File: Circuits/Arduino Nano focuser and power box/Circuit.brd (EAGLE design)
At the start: 67.4 x 71.6 mm, 30 parts, among them IC1 7805L, J2 RJ11, Q2 IRF540, Q3 IRF540, Q5 BC547

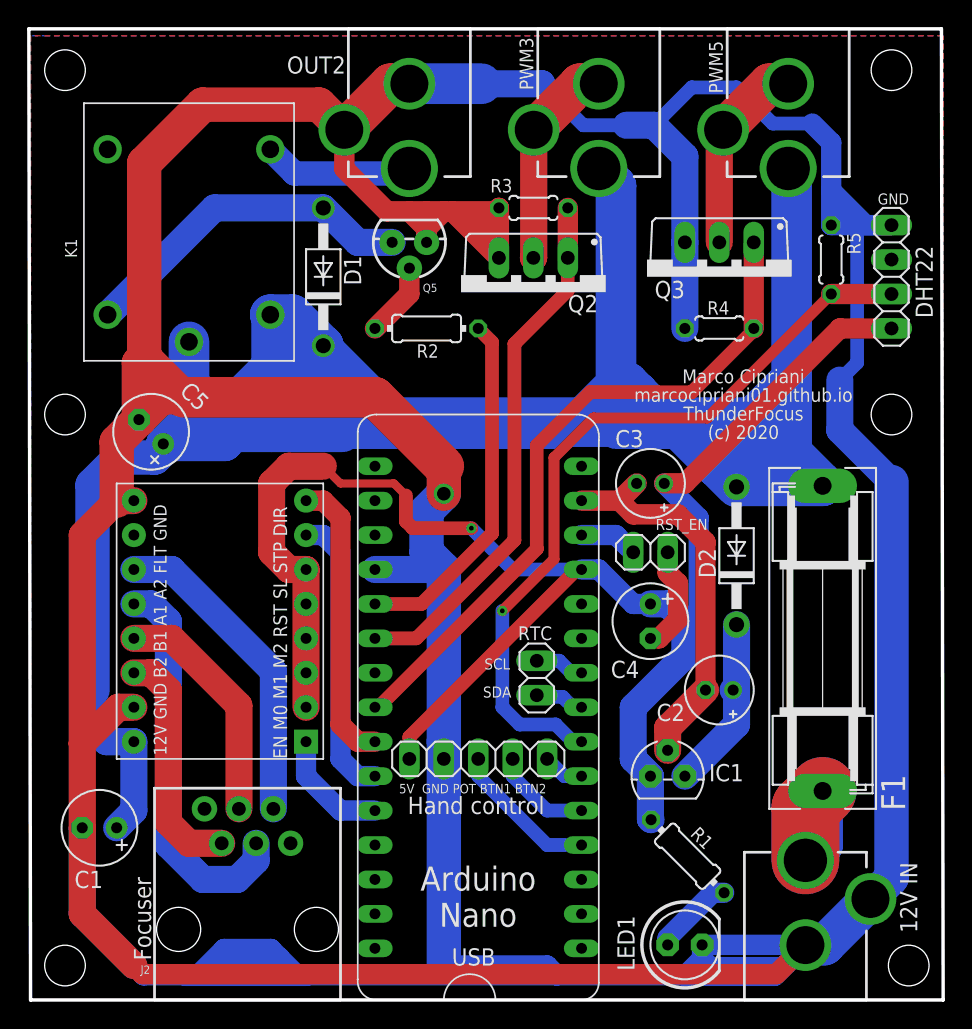
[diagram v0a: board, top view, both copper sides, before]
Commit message: Update files
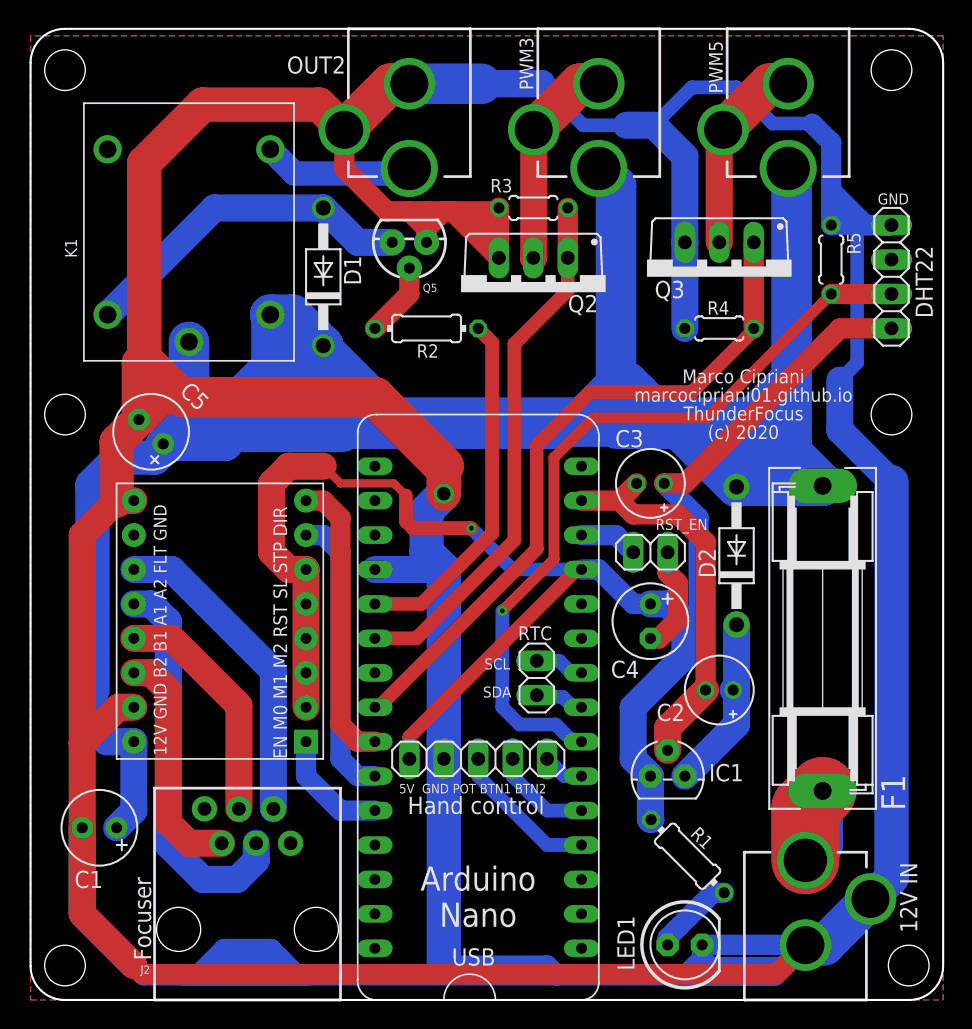
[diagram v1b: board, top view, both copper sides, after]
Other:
- board size 67.4 x 71.6 mm -> 67.3 x 71.6 mm
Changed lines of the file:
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@@
 <drawing>
 <settings>
-<setting alwaysvectorfont="yes"/>
+<setting alwaysvectorfont="no"/>
 <setting verticaltext="up"/>
 </settings>
@@
 <hole x="63.5" y="68.58" drill="3"/>
 <hole x="2.54" y="68.58" drill="3"/>
-<wire x1="0" y1="0" x2="67.31" y2="0" width="0.254" layer="20"/>
-<wire x1="67.31" y1="0" x2="67.183" y2="71.628" width="0.254" layer="20"/>
-<wire x1="67.183" y1="71.628" x2="-0.127" y2="71.628" width="0.254" layer="20"/>
-<wire x1="-0.127" y1="71.628" x2="0" y2="0" width="0.254" layer="20"/>
 <text x="10.033" y="18.034" size="0.95" layer="25" distance="37" rot="R90">12V GND B2 B1 A1 A2 FLT GND</text>
 <text x="18.923" y="17.78" size="1.016" layer="25" distance="26" rot="R90">EN M0 M1 M2 RST SL STP DIR</text>
@@
 SDA</text>
 <text x="37.211" y="27.051" size="1.016" layer="21" distance="155" align="center">RTC</text>
+<wire x1="2.5" y1="0" x2="64.81" y2="0" width="0.1524" layer="20"/>
+<wire x1="64.81" y1="0" x2="67.31" y2="2.5" width="0.1524" layer="20" curve="90"/>
+<wire x1="67.31" y1="2.5" x2="67.31" y2="69.128" width="0.1524" layer="20"/>
+<wire x1="67.31" y1="69.128" x2="64.81" y2="71.628" width="0.1524" layer="20" curve="90"/>
+<wire x1="64.81" y1="71.628" x2="2.5" y2="71.628" width="0.1524" layer="20"/>
+<wire x1="2.5" y1="71.628" x2="0" y2="69.128" width="0.1524" layer="20" curve="90"/>
+<wire x1="0" y1="69.128" x2="0" y2="2.5" width="0.1524" layer="20"/>
+<wire x1="0" y1="2.5" x2="2.5" y2="0" width="0.1524" layer="20" curve="90"/>
 </plain>
 <attributes>
@@
 <vertex x="67.31" y="0"/>
 <vertex x="67.31" y="71.12"/>
-<vertex x="1.27" y="71.12"/>
 </polygon>
 <polygon width="1.5" layer="1" isolate="0.6096">
